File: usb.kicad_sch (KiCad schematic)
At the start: 122 parts, among them J4 WE_632723300011_alt_symbol, U10 TUSB1046-DCI, U12 AP22615, U13 TPD4E05U06QDQARQ1, U14 TPD4E05U06QDQARQ1, U15 TPD4E05U06QDQARQ1, U16 TPD4E05U06QDQARQ1, U5 FT230XQ-R, U6 TPS65988, U7 W25Q80DVUXIE_TR, U8 NCP730BMT330TBG

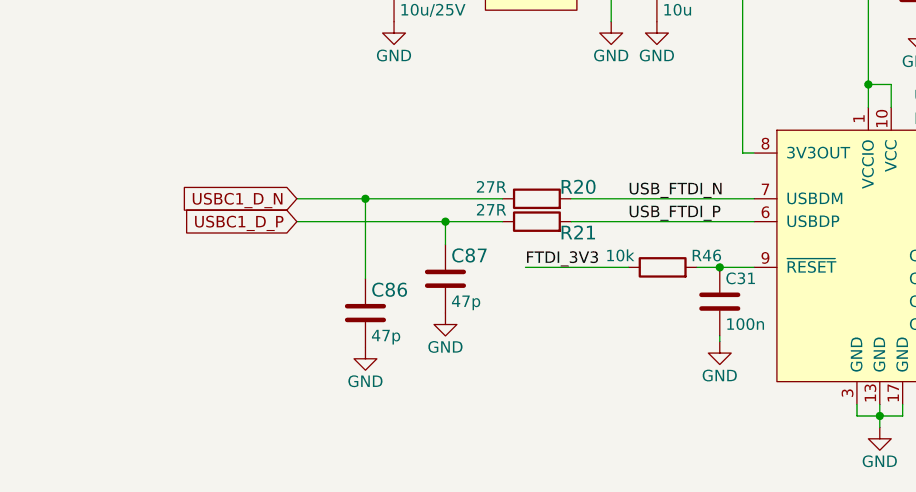
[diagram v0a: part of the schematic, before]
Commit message: Small changes
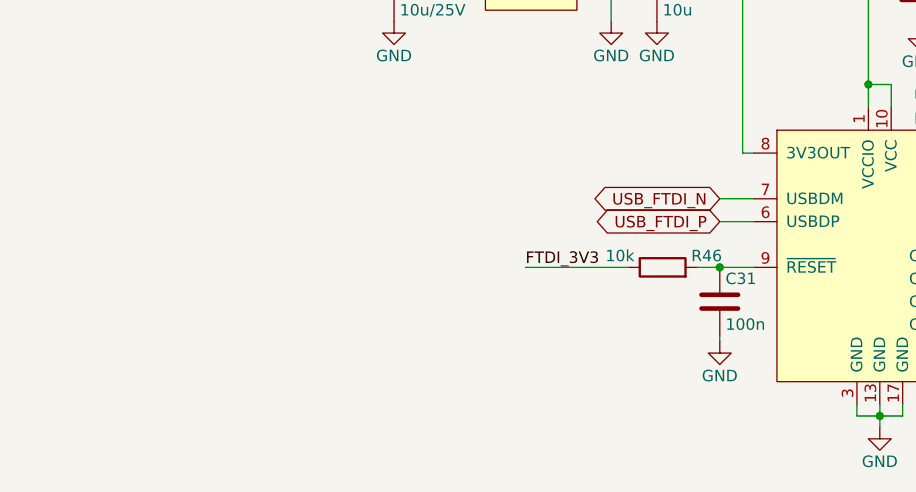
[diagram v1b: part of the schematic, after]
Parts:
- removed C86, C87: C_47p_0402, jetson-orin-baseboard-footprints:0402-cap, symbol jetson-orin-baseboard:C_47p_0402
- removed R20, R21: R_27R_0402, jetson-orin-baseboard-footprints:0402-res, symbol jetson-orin-baseboard:R_27R_0402
